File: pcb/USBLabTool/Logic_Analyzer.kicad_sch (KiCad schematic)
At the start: 20 parts, among them U18 74HC245, U20 74HC245

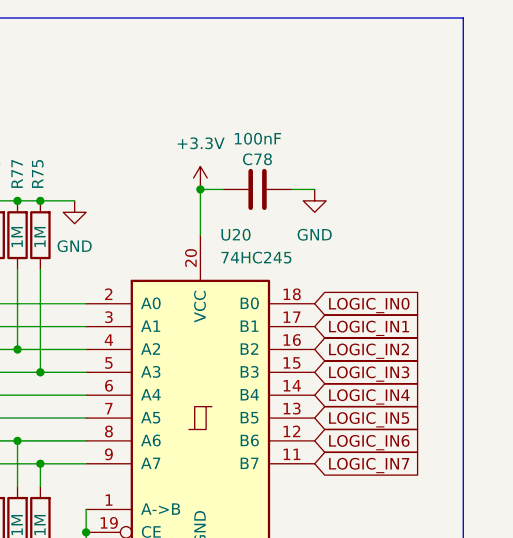
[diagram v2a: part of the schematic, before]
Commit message: merge from V2
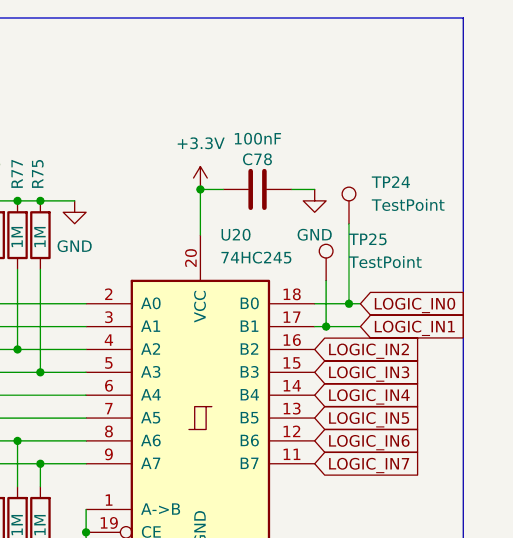
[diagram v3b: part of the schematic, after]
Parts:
- added TP24, TP25: TestPoint, TestPoint:TestPoint_Pad_2.0x2.0mm, symbol Connector:TestPoint
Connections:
- net LOGIC_IN0: now also TP24.1
- net LOGIC_IN1: now also TP25.1
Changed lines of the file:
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@@
 	)
 	(junction
+		(at 207.01 77.47)
+		(diameter 0)
+		(color 0 0 0 0)
+	)
+	(junction
 		(at 85.09 74.93)
 		(diameter 0)
@@
 	)
 	(junction
+		(at 209.55 74.93)
+		(diameter 0)
+		(color 0 0 0 0)
+	)
+	(junction
 		(at 87.63 104.14)
 		(diameter 0)
@@
 	(wire
 		(pts
+			(xy 207.01 72.39) (xy 207.01 77.47)
+		)
+		(stroke
+			(width 0)
+			(type default)
+		)
+	)
+	(wire
+		(pts
 			(xy 166.37 85.09) (xy 167.64 85.09)
 		)
@@
 	(wire
 		(pts
+			(xy 210.82 74.93) (xy 209.55 74.93)
+		)
+		(stroke
+			(width 0)
+			(type default)
+		)
+	)
+	(wire
+		(pts
 			(xy 85.09 85.09) (xy 85.09 96.52)
 		)
@@
 	(wire
 		(pts
+			(xy 205.74 74.93) (xy 209.55 74.93)
+		)
+		(stroke
+			(width 0)
+			(type default)
+		)
+	)
+	(wire
+		(pts
 			(xy 83.82 85.09) (xy 85.09 85.09)
 		)
@@
 	(wire
 		(pts
+			(xy 210.82 77.47) (xy 207.01 77.47)
+		)
+		(stroke
+			(width 0)
+			(type default)
+		)
+	)
+	(wire
+		(pts
 			(xy 172.72 102.87) (xy 175.26 102.87)
 		)
@@
 	(wire
 		(pts
+			(xy 207.01 77.47) (xy 205.74 77.47)
+		)
+		(stroke
+			(width 0)
+			(type default)
+		)
+	)
+	(wire
+		(pts
 			(xy 83.82 92.71) (xy 92.71 92.71)
 		)
@@
 	(wire
 		(pts
+			(xy 209.55 66.04) (xy 209.55 74.93)
+		)
+		(stroke
+			(width 0)
+			(type default)
+		)
+	)
+	(wire
+		(pts
 			(xy 175.26 92.71) (xy 180.34 92.71)
 		)
@@
 	(global_label "LOGIC_IN0"
 		(shape input)
-		(at 205.74 74.93 0)
+		(at 210.82 74.93 0)
 		(fields_autoplaced yes)
 		(effects
@@
 		)
 		(property "Intersheetrefs" "${INTERSHEET_REFS}"
-			(at 218.341 74.93 0)
+			(at 223.421 74.93 0)
 			(effects
 				(font
@@
 	(global_label "LOGIC_IN1"
 		(shape input)
-		(at 205.74 77.47 0)
+		(at 210.82 77.47 0)
 		(fields_autoplaced yes)
 		(effects
@@
 		)
 		(property "Intersheetrefs" "${INTERSHEET_REFS}"
-			(at 218.341 77.47 0)
+			(at 223.421 77.47 0)
 			(effects
 				(font
@@
 	)
 	(symbol
+		(lib_id "Connector:TestPoint")
+		(at 207.01 72.39 0)
+		(unit 1)
+		(exclude_from_sim no)
+		(in_bom yes)
+		(on_board yes)
+		(dnp no)
+		(fields_autoplaced yes)
+		(property "Reference" "TP25"
+			(at 209.55 67.8179 0)
+			(effects
+				(font
+					(size 1.27 1.27)
+				)
+				(justify left)
+			)
+		)
+		(property "Value" "TestPoint"
+			(at 209.55 70.3579 0)
+			(effects
+				(font
+					(size 1.27 1.27)
+				)
+				(justify left)
+			)
+		)
+		(property "Footprint" "TestPoint:TestPoint_Pad_2.0x2.0mm"
+			(at 212.09 72.39 0)
+			(effects
+				(font
+					(size 1.27 1.27)
+				)
+				(hide yes)
+			)
+		)
+		(property "Datasheet" "~"
+			(at 212.09 72.39 0)
+			(effects
+				(font
+					(size 1.27 1.27)
+				)
+				(hide yes)
+			)
+		)
+		(property "Description" "test point"
+			(at 207.01 72.39 0)
+			(effects
+				(font
+					(size 1.27 1.27)
+				)
+				(hide yes)
+			)
+		)
+		(pin "1"
+		)
+		(instances
+			(project ""
+				(path "/b5440f7d-90d5-417e-adc2-aa6b11e5424d/a25b8bd5-b6d2-402d-8b42-7856aa781e02"
+					(reference "TP25")
+					(unit 1)
+				)
+			)
+		)
+	)
+	(symbol
 		(lib_id "Device:R")
 		(at 87.63 100.33 180)
@@
 					(unit 1)
 				)
+			)
+		)
+	)
+	(symbol
+		(lib_id "Connector:TestPoint")
+		(at 209.55 66.04 0)
+		(unit 1)
+		(exclude_from_sim no)
+		(in_bom yes)
+		(on_board yes)
+		(dnp no)
+		(fields_autoplaced yes)
+		(property "Reference" "TP24"
+			(at 212.09 61.4679 0)
+			(effects
+				(font
+					(size 1.27 1.27)
+				)
+				(justify left)
+			)
+		)
+		(property "Value" "TestPoint"
+			(at 212.09 64.0079 0)
+			(effects
+				(font
+					(size 1.27 1.27)
+				)
+				(justify left)
+			)
+		)
+		(property "Footprint" "TestPoint:TestPoint_Pad_2.0x2.0mm"
+			(at 214.63 66.04 0)
+			(effects
+				(font
+					(size 1.27 1.27)
+				)
+				(hide yes)
+			)
+		)
+		(property "Datasheet" "~"
+			(at 214.63 66.04 0)
+			(effects
+				(font
+					(size 1.27 1.27)
+				)
+				(hide yes)
+			)
+		)
+		(property "Description" "test point"
+			(at 209.55 66.04 0)
+			(effects
+				(font
+					(size 1.27 1.27)
+				)
+				(hide yes)
+			)
+		)
+		(pin "1"
+		)
+		(instances
+			(project ""
+				(path "/b5440f7d-90d5-417e-adc2-aa6b11e5424d/a25b8bd5-b6d2-402d-8b42-7856aa781e02"
+					(reference "TP24")
+					(unit 1)
+				)
